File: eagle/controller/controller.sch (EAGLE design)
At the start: 35 parts, among them IC1 ATMEGA48/88/168-PU, K1 REED, K2 REED, K3 REED, Q1 BC517, Q2 BC517, Q3 BC517, X1 43160-1102, X2 43160-1102, X3 43160-1102, X5 C-GRID-02-15-19

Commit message: Complete the circuit
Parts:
- added B4: (no value), e-messfuehler:MESSFUEHLER_2
- added F2: (no value), e-sicherungen:SICHERUNG_1-POL
- added POWER230V1: C-GRID-02-15-19, con-molex:C-GRID-02-15-19
- added Q4: BC517, transistor-npn:BC517
- added R12, R13: 1M, resistor:R-EU_0204/7
- added R14, R15: 10k, resistor:R-EU_0204/7
- added X6: 43160-1102, con-molex:43160-1102
- K1, K2: value REED -> (none); device relay:REED -> e-schuetze-relais:HILFSSCHUETZ_13-14; TYPE (none) -> JS 05 MN KT
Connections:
- removed net N$3 (its old number): IC4.O3, K11.-
- new net N$18: IC1.PD3(INT1/OC2B/PCINT19), Q4.C, R14.1
- new net N$31: IC4.O2, K2G$1.A2
- new net N$33: F2.2
- new net N$34: F2.1, POWER230V1-1.S
- new net N$35: K21.4, POWER230V1-2.S
- new net N$5: B4.1
- net GND: now also Q4.E, R15.1
- net N$1: now also K1G$1.A2
- net N$10: now also X6-1.S@2; no longer K22.P, X2-2.S@1
- net N$11: now also Q4.B, R13.1, R15.2; no longer K12.P, X3-2.S@1
- net N$12: now also R12.1
- net N$17: now also R12.2
- net N$4: now also B4.2; no longer IC4.O2, K21.-
- net N$9: now also X2-2.S@1, X3-2.S@1, X6-2.S@1
- net VCC: now also K1G$1.A1, K2G$1.A1, R14.2; no longer K11.+, K12.S, K21.+, K22.S
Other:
- moved on the sheet: F1, K6, R2, R3, R4, R5, R6, R7

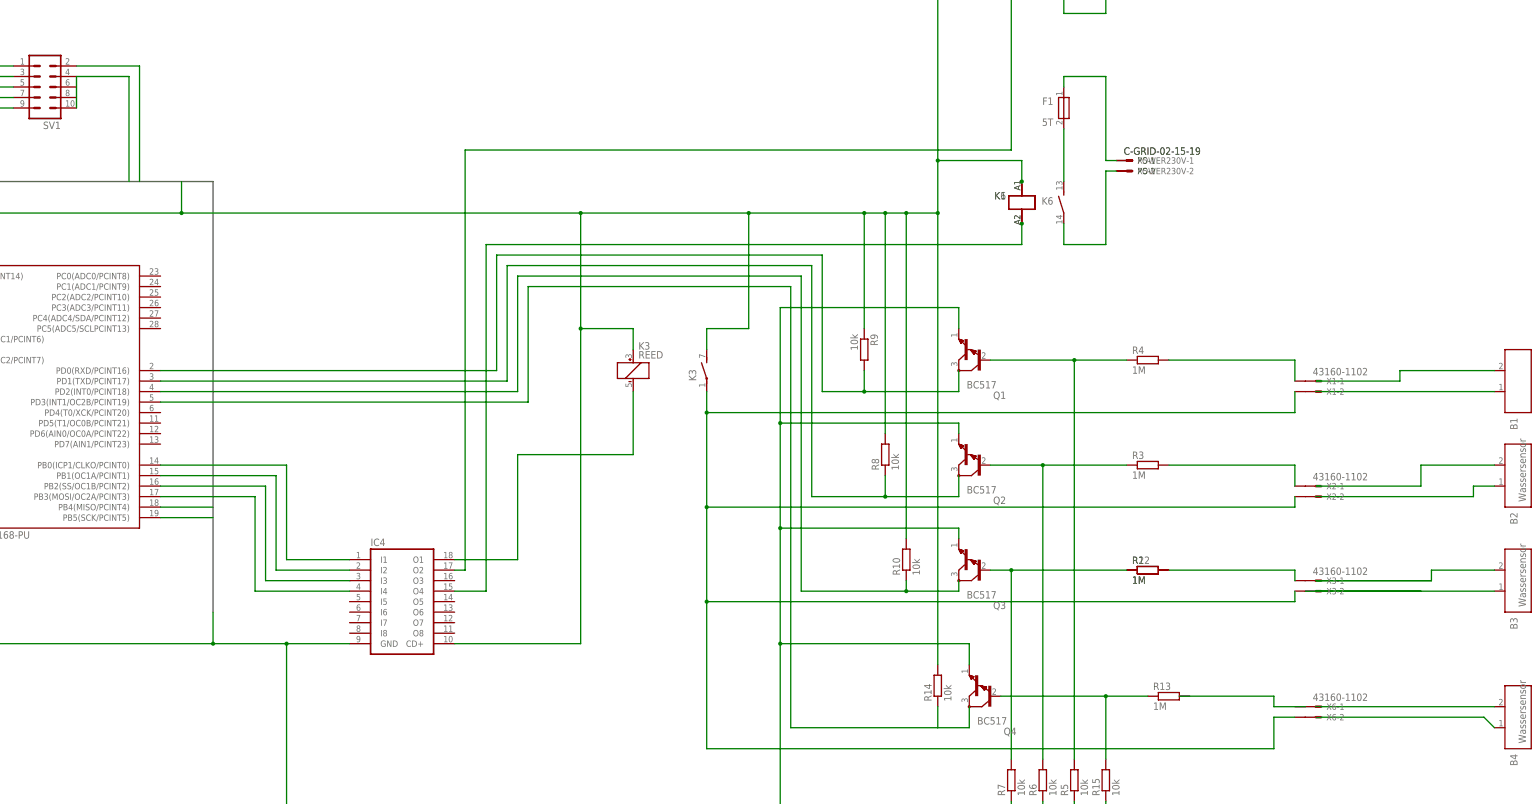
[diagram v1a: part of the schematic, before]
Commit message: corrected errors
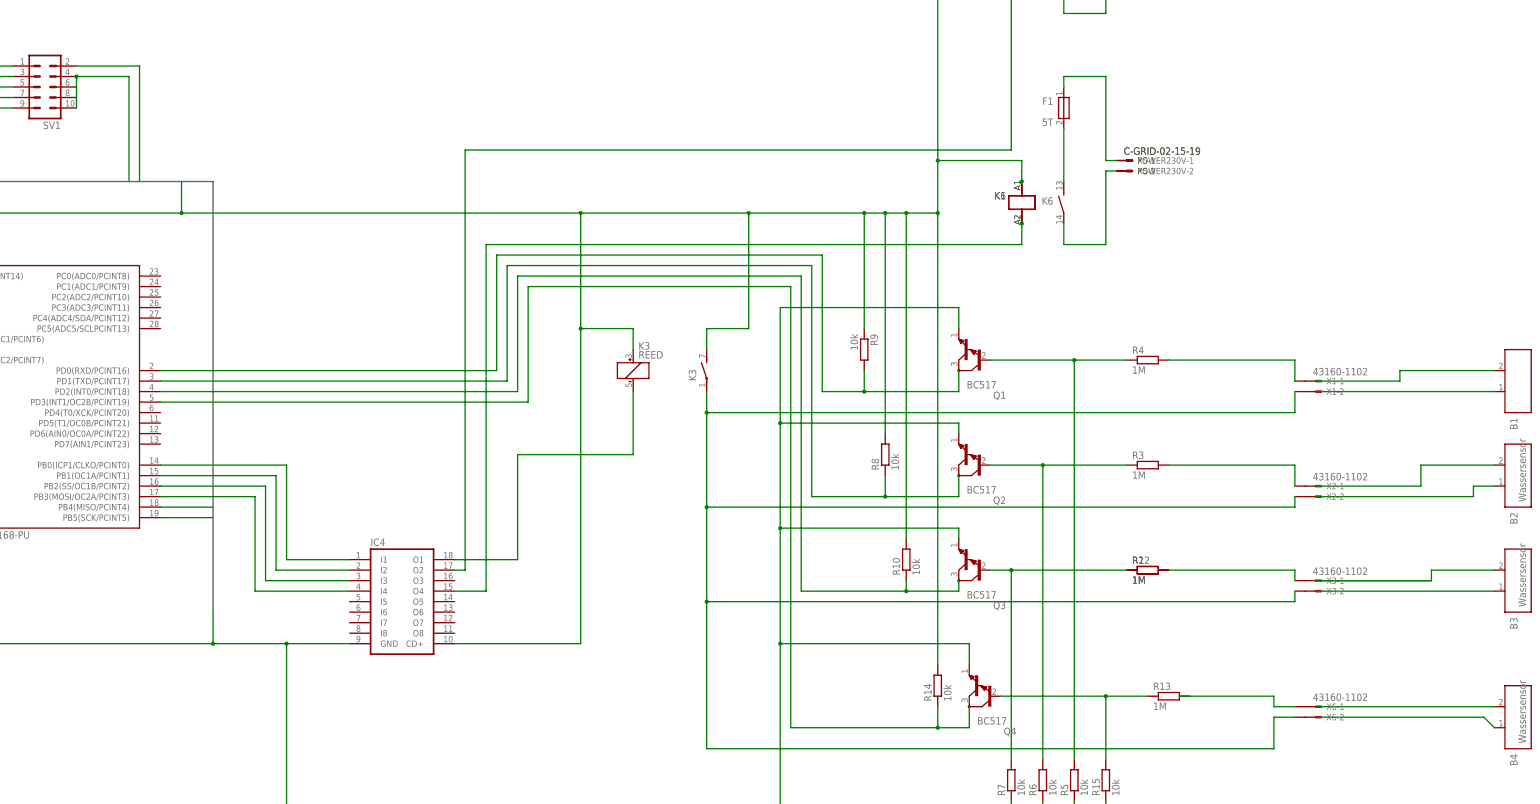
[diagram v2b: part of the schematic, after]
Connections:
- net N$10: now also X6-1.S@1; no longer X6-1.S@2
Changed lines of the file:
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@@
 <wire x1="353.06" y1="7.62" x2="381" y2="7.62" width="0.1524" layer="91"/>
-</segment>
-<segment>
-<wire x1="350.52" y1="5.08" x2="378.46" y2="5.08" width="0.1524" layer="91"/>
-</segment>
-</net>
-<net name="N$27" class="0">
-<segment>
-<pinref part="B3" gate="G$1" pin="1"/>
-<wire x1="353.06" y1="5.08" x2="396.24" y2="5.08" width="0.1524" layer="91"/>
 </segment>
 </net>
@@
 <pinref part="SV1" gate="G$1" pin="10"/>
 <wire x1="53.34" y1="121.92" x2="53.34" y2="129.54" width="0.1524" layer="91"/>
+<junction x="53.34" y="129.54"/>
 </segment>
 <segment>
@@
 <pinref part="R14" gate="G$1" pin="1"/>
 <wire x1="261.62" y1="-27.94" x2="261.62" y2="-22.86" width="0.1524" layer="91"/>
+<junction x="261.62" y="-27.94"/>
 </segment>
 </net>
 <net name="N$10" class="0">
 <segment>
-<pinref part="X6" gate="-1" pin="S@2"/>
-<wire x1="350.52" y1="-22.86" x2="342.9" y2="-22.86" width="0.1524" layer="91"/>
 <wire x1="342.9" y1="-22.86" x2="342.9" y2="-20.32" width="0.1524" layer="91"/>
 <wire x1="342.9" y1="-20.32" x2="320.04" y2="-20.32" width="0.1524" layer="91"/>
+<pinref part="X6" gate="-1" pin="S@1"/>
+<wire x1="347.98" y1="-22.86" x2="342.9" y2="-22.86" width="0.1524" layer="91"/>
 </segment>
 </net>
@@
 </segment>
 </net>
+<net name="N$27" class="0">
+<segment>
+<pinref part="B3" gate="G$1" pin="1"/>
+<wire x1="396.24" y1="5.08" x2="353.06" y2="5.08" width="0.1524" layer="91"/>
+</segment>
+</net>
